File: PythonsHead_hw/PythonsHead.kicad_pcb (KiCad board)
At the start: 2 copper layers, 45 x 79.5 mm, 92 parts, among them Q1 MMBT2222, Q2 MMBT2222, Q3 MMBT2222, Q4 MMBT2222, Q5 MMBT2222, Q6 MMBT2222, Q7 MMBT2222, Q8 MMBT2222

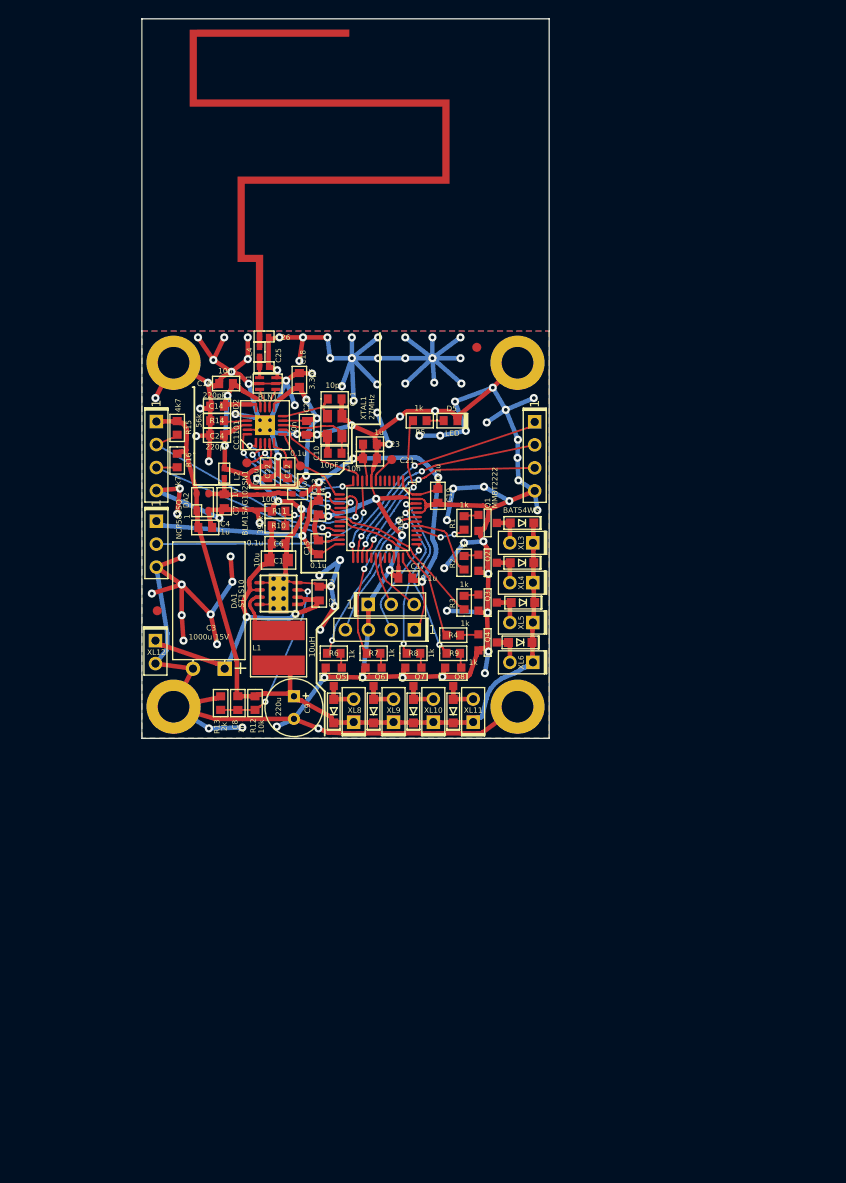
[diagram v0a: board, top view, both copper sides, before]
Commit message: Layout done
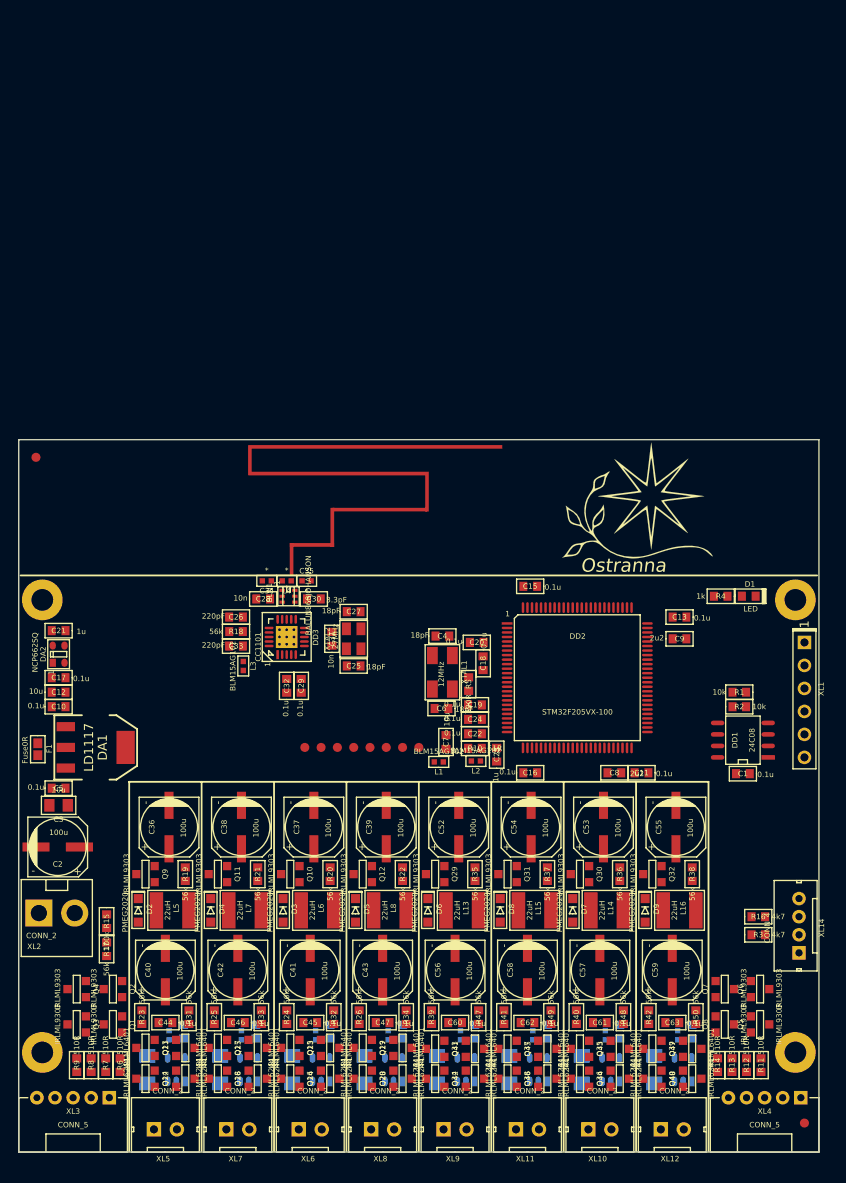
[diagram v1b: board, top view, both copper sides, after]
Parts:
- removed C14: 220pF, Capacitors:CAP_0603
- removed XL13: CONN_3, Connectors:PLS-3
- added C27: 18pF, Capacitors:CAP_0603, F.Cu at (115.4, 85.0)
- added C28: 10n, Capacitors:CAP_0603, F.Cu at (105.4, 83.6)
- added C29: 0.1u, Capacitors:CAP_0603, F.Cu at (109.6, 93.2)
- added C30: 3.3pF, Capacitors:CAP_0603, F.Cu at (111.0, 83.6)
- added C31: 10n, Capacitors:CAP_0603, F.Cu at (113.0, 88.0)
- added C32: 0.1u, Capacitors:CAP_0603, F.Cu at (108.0, 93.2)
- added C33: 220pF, Capacitors:CAP_0603, F.Cu at (102.4, 88.8)
- added C34: *, Capacitors:CAP_0402, F.Cu at (105.8, 81.6)
- added C35: *, Capacitors:CAP_0402, F.Cu at (110.2, 81.6)
- added C36: 100u, Capacitors:SMD_D6d3, F.Cu at (95.0, 108.8)
- added C37: 100u, Capacitors:SMD_D6d3, F.Cu at (111.0, 108.8)
- added C38: 100u, Capacitors:SMD_D6d3, F.Cu at (103.0, 108.8)
- added C39: 100u, Capacitors:SMD_D6d3, F.Cu at (119.0, 108.8)
- added C40: 100u, Capacitors:SMD_D6d3, F.Cu at (94.6, 124.6)
- added C41: 100u, Capacitors:SMD_D6d3, F.Cu at (110.6, 124.6)
- added C42: 100u, Capacitors:SMD_D6d3, F.Cu at (102.6, 124.6)
- added C43: 100u, Capacitors:SMD_D6d3, F.Cu at (118.6, 124.6)
- added C44: 0.1u, Capacitors:CAP_0603, F.Cu at (94.6, 130.4)
- added C45: 0.1u, Capacitors:CAP_0603, F.Cu at (110.6, 130.4)
- added C46: 0.1u, Capacitors:CAP_0603, F.Cu at (102.6, 130.4)
- added C47: 0.1u, Capacitors:CAP_0603, F.Cu at (118.6, 130.4)
- added C48: 0.1u, Capacitors:CAP_0603, B.Cu at (96.6, 131.4)
- added C49: 0.1u, Capacitors:CAP_0603, B.Cu at (112.8, 131.4)
- added C5: 0.1u, Capacitors:CAP_0603, F.Cu at (82.8, 104.5)
- added C50: 0.1u, Capacitors:CAP_0603, B.Cu at (104.6, 131.4)
- added C51: 0.1u, Capacitors:CAP_0603, B.Cu at (120.8, 131.4)
- added C52: 100u, Capacitors:SMD_D6d3, F.Cu at (127.0, 108.8)
- added C53: 100u, Capacitors:SMD_D6d3, F.Cu at (143.0, 108.8)
- added C54: 100u, Capacitors:SMD_D6d3, F.Cu at (135.0, 108.8)
- added C55: 100u, Capacitors:SMD_D6d3, F.Cu at (151.0, 108.8)
- added C56: 100u, Capacitors:SMD_D6d3, F.Cu at (126.6, 124.6)
- added C57: 100u, Capacitors:SMD_D6d3, F.Cu at (142.6, 124.6)
- added C58: 100u, Capacitors:SMD_D6d3, F.Cu at (134.6, 124.6)
- added C59: 100u, Capacitors:SMD_D6d3, F.Cu at (150.6, 124.6)
- added C60: 0.1u, Capacitors:CAP_0603, F.Cu at (126.6, 130.4)
- added C61: 0.1u, Capacitors:CAP_0603, F.Cu at (142.6, 130.4)
- added C62: 0.1u, Capacitors:CAP_0603, F.Cu at (134.6, 130.4)
- added C63: 0.1u, Capacitors:CAP_0603, F.Cu at (150.6, 130.4)
- added C64: 0.1u, Capacitors:CAP_0603, B.Cu at (128.8, 131.4)
- added C65: 0.1u, Capacitors:CAP_0603, B.Cu at (144.8, 131.4)
- added C66: 0.1u, Capacitors:CAP_0603, B.Cu at (136.8, 131.4)
- added C67: 0.1u, Capacitors:CAP_0603, B.Cu at (152.8, 131.4)
- added DA10: AD8211, SOT:SOT23-5, B.Cu at (151.8, 135.6)
- added DA3: AD8211, SOT:SOT23-5, B.Cu at (95.8, 135.6)
- added DA4: AD8211, SOT:SOT23-5, B.Cu at (111.8, 135.6)
- added DA5: AD8211, SOT:SOT23-5, B.Cu at (103.8, 135.6)
- added DA6: AD8211, SOT:SOT23-5, B.Cu at (119.8, 135.6)
- added DA7: AD8211, SOT:SOT23-5, B.Cu at (127.8, 135.6)
- added DA8: AD8211, SOT:SOT23-5, B.Cu at (143.8, 135.6)
- added DA9: AD8211, SOT:SOT23-5, B.Cu at (135.8, 135.6)
- added DD3: CC1101, QFN_DFN:QFN20, F.Cu at (108.0, 87.8)
- added F1: Fuse0R, Resistors:RES_0603_FUSE, F.Cu at (80.5, 100.2)
- added L10: BLM15AG102, Inductors:IND_0402, B.Cu at (111.2, 131.8)
- added L11: BLM15AG102, Inductors:IND_0402, B.Cu at (103.0, 131.8)
- added L12: BLM15AG102, Inductors:IND_0402, B.Cu at (119.2, 131.8)
- added L13: 22uH, Inductors:SRN5040, F.Cu at (127.4, 118.0)
- added L14: 22uH, Inductors:SRN5040, F.Cu at (143.4, 118.0)
- added L15: 22uH, Inductors:SRN5040, F.Cu at (135.4, 118.0)
- added L16: 22uH, Inductors:SRN5040, F.Cu at (151.4, 118.0)
- added L17: BLM15AG102, Inductors:IND_0402, B.Cu at (127.2, 131.8)
- added L18: BLM15AG102, Inductors:IND_0402, B.Cu at (143.2, 131.8)
- added L19: BLM15AG102, Inductors:IND_0402, B.Cu at (135.2, 131.8)
- added L20: BLM15AG102, Inductors:IND_0402, B.Cu at (151.2, 131.8)
- added L5: 22uH, Inductors:SRN5040, F.Cu at (95.4, 118.0)
- added L6: 22uH, Inductors:SRN5040, F.Cu at (111.4, 118.0)
- added L7: 22uH, Inductors:SRN5040, F.Cu at (103.4, 118.0)
- added L8: 22uH, Inductors:SRN5040, F.Cu at (119.4, 118.0)
- added L9: BLM15AG102, Inductors:IND_0402, B.Cu at (95.0, 131.8)
- added Logo1: Logo, Pictures:Ostranna_16d9_13d5, F.Cu at (146.7, 72.7)
- added Q10: IRLML9303, SOT:SOT23-3, F.Cu at (108.4, 114.0)
- added Q11: IRLML9303, SOT:SOT23-3, F.Cu at (100.4, 114.0)
- added Q12: IRLML9303, SOT:SOT23-3, F.Cu at (116.4, 114.0)
- added Q13: IRLML6401, SOT:SOT23-3, F.Cu at (92.4, 133.2)
- added Q14: IRLML6244, SOT:SOT23-3, F.Cu at (92.4, 136.6)
- added Q15: IRLML6401, SOT:SOT23-3, F.Cu at (108.4, 133.2)
- added Q16: IRLML6244, SOT:SOT23-3, F.Cu at (108.4, 136.6)
- added Q17: IRLML6401, SOT:SOT23-3, F.Cu at (100.4, 133.2)
- added Q18: IRLML6244, SOT:SOT23-3, F.Cu at (100.4, 136.6)
- added Q19: IRLML6401, SOT:SOT23-3, F.Cu at (116.4, 133.2)
- added Q20: IRLML6244, SOT:SOT23-3, F.Cu at (116.4, 136.6)
- added Q21: IRLML6401, SOT:SOT23-3, F.Cu at (96.8, 133.2)
- added Q22: IRLML6244, SOT:SOT23-3, F.Cu at (96.8, 136.6)
- added Q23: IRLML6401, SOT:SOT23-3, F.Cu at (112.8, 133.2)
- added Q24: IRLML6244, SOT:SOT23-3, F.Cu at (112.8, 136.6)
- added Q25: IRLML6401, SOT:SOT23-3, F.Cu at (104.8, 133.2)
- added Q26: IRLML6244, SOT:SOT23-3, F.Cu at (104.8, 136.6)
- added Q27: IRLML6401, SOT:SOT23-3, F.Cu at (120.8, 133.2)
- added Q28: IRLML6244, SOT:SOT23-3, F.Cu at (120.8, 136.6)
- added Q29: IRLML9303, SOT:SOT23-3, F.Cu at (124.4, 114.0)
- added Q30: IRLML9303, SOT:SOT23-3, F.Cu at (140.4, 114.0)
- added Q31: IRLML9303, SOT:SOT23-3, F.Cu at (132.4, 114.0)
- added Q32: IRLML9303, SOT:SOT23-3, F.Cu at (148.4, 114.0)
- added Q33: IRLML6401, SOT:SOT23-3, F.Cu at (124.4, 133.3)
- added Q34: IRLML6244, SOT:SOT23-3, F.Cu at (124.4, 136.6)
- added Q35: IRLML6401, SOT:SOT23-3, F.Cu at (140.4, 133.3)
- added Q36: IRLML6244, SOT:SOT23-3, F.Cu at (140.4, 136.6)
- added Q37: IRLML6401, SOT:SOT23-3, F.Cu at (132.4, 133.3)
- added Q38: IRLML6244, SOT:SOT23-3, F.Cu at (132.4, 136.6)
- added Q39: IRLML6401, SOT:SOT23-3, F.Cu at (148.4, 133.3)
- added Q40: IRLML6244, SOT:SOT23-3, F.Cu at (148.4, 136.6)
- added Q41: IRLML6401, SOT:SOT23-3, F.Cu at (128.8, 133.3)
- added Q42: IRLML6244, SOT:SOT23-3, F.Cu at (128.8, 136.6)
- added Q43: IRLML6401, SOT:SOT23-3, F.Cu at (144.8, 133.3)
- added Q44: IRLML6244, SOT:SOT23-3, F.Cu at (144.8, 136.6)
- added Q45: IRLML6401, SOT:SOT23-3, F.Cu at (136.8, 133.3)
- added Q46: IRLML6244, SOT:SOT23-3, F.Cu at (136.8, 136.6)
- added Q47: IRLML6401, SOT:SOT23-3, F.Cu at (152.8, 133.3)
- added Q48: IRLML6244, SOT:SOT23-3, F.Cu at (152.8, 136.6)
- added Q9: IRLML9303, SOT:SOT23-3, F.Cu at (92.4, 114.0)
- added R17: 56k, Resistors:RES_0603, F.Cu at (88.1, 122.3)
- added R18: 56k, Resistors:RES_0603, F.Cu at (102.4, 87.2)
- added R19: 56k, Resistors:RES_0603, F.Cu at (96.8, 114.0)
- added R20: 56k, Resistors:RES_0603, F.Cu at (112.8, 114.0)
- added R21: 56k, Resistors:RES_0603, F.Cu at (104.8, 114.0)
- added R22: 56k, Resistors:RES_0603, F.Cu at (120.8, 114.0)
- added R23: 56k, Resistors:RES_0603, F.Cu at (92.0, 129.8)
- added R24: 56k, Resistors:RES_0603, F.Cu at (108.0, 129.8)
- added R25: 56k, Resistors:RES_0603, F.Cu at (100.0, 129.8)
- added R26: 56k, Resistors:RES_0603, F.Cu at (116.0, 129.8)
- added R27: 0R1, Resistors:RES_1206, B.Cu at (92.6, 135.6)
- added R28: 0R1, Resistors:RES_1206, B.Cu at (108.6, 135.6)
- added R29: 0R1, Resistors:RES_1206, B.Cu at (100.7, 135.6)
- added R30: 0R1, Resistors:RES_1206, B.Cu at (116.6, 135.6)
- added R31: 56k, Resistors:RES_0603, F.Cu at (97.2, 129.8)
- added R32: 56k, Resistors:RES_0603, F.Cu at (113.2, 129.8)
- added R33: 56k, Resistors:RES_0603, F.Cu at (105.2, 129.8)
- added R34: 56k, Resistors:RES_0603, F.Cu at (121.2, 129.8)
- added R35: 56k, Resistors:RES_0603, F.Cu at (128.8, 114.0)
- added R36: 56k, Resistors:RES_0603, F.Cu at (144.8, 114.0)
- added R37: 56k, Resistors:RES_0603, F.Cu at (136.8, 114.0)
- added R38: 56k, Resistors:RES_0603, F.Cu at (152.8, 114.0)
- added R39: 56k, Resistors:RES_0603, F.Cu at (124.0, 129.8)
- added R40: 56k, Resistors:RES_0603, F.Cu at (140.0, 129.8)
- added R41: 56k, Resistors:RES_0603, F.Cu at (132.0, 129.8)
- added R42: 56k, Resistors:RES_0603, F.Cu at (148.0, 129.8)
- added R43: 0R1, Resistors:RES_1206, B.Cu at (124.6, 135.6)
- added R44: 0R1, Resistors:RES_1206, B.Cu at (140.6, 135.6)
- added R45: 0R1, Resistors:RES_1206, B.Cu at (132.6, 135.6)
- added R46: 0R1, Resistors:RES_1206, B.Cu at (148.6, 135.6)
- added R47: 56k, Resistors:RES_0603, F.Cu at (129.2, 129.8)
- added R48: 56k, Resistors:RES_0603, F.Cu at (145.2, 129.8)
- added R49: 56k, Resistors:RES_0603, F.Cu at (137.2, 129.8)
- added R50: 56k, Resistors:RES_0603, F.Cu at (153.2, 129.8)
- added TP4: TESTPOINT, PCB:TESTPOINT_1MM, F.Cu at (115.4, 100.0)
- added TP5: TESTPOINT, PCB:TESTPOINT_1MM, F.Cu at (117.2, 100.0)
- added TP6: TESTPOINT, PCB:TESTPOINT_1MM, F.Cu at (120.8, 100.0)
- added TP7: TESTPOINT, PCB:TESTPOINT_1MM, F.Cu at (119.0, 100.0)
- added TP8: TESTPOINT, PCB:TESTPOINT_1MM, F.Cu at (122.6, 100.0)
- added XTAL2: 27MHz, Quartz:03225C4, F.Cu at (115.4, 88.0)
- ANT1: footprint Radio:ANT_868_MEANDER_4HOR_45mm -> Radio:ANT_868_ARMLETG
- BLN1: value 0896BM15A0001 -> BALUN868JOHANSON
- C1: value 10u -> 0.1u; footprint Capacitors:CAP_0805 -> Capacitors:CAP_0603
- C10, C11: value 10pF -> 0.1u
- C12: value 0.1u -> 10u
- C13: value 4.7u -> 0.1u
- C16, C20: value 10n -> 0.1u
- C18: value 3.3pF -> 0.1u
- C2: value 1u -> 100u; footprint Capacitors:CAP_0603 -> Capacitors:SMD_D6d3
- C21: value 10n -> 1u
- C24: value 220pF -> 0.1u
- C25: value 1.5pF -> 18pF; footprint Capacitors:CAP_0402 -> Capacitors:CAP_0603
- C26: value DoNotMount -> 220pF; footprint Capacitors:CAP_0402 -> Capacitors:CAP_0603
- C3: value 1000u 15V -> 10u; footprint Capacitors:CAP_08xxR_HOR -> Capacitors:CAP_0805
- C4: value 1u -> 18pF
- C6: value 0.1u -> 18pF
- C7: value 1u -> 10u
- C8: value 1n -> 2u2
- C9: value 220u -> 2u2; footprint Capacitors:CAP_06xxR -> Capacitors:CAP_0603
- D1: value BAT54WS -> LED; footprint Diodes:SOD323 -> LEDs:LED_0603
- D2, D3, D4, D6, D7, D8, D9: value BAT54WS -> PMEG2020
- D5: value LED -> PMEG2020; footprint LEDs:LED_0603 -> Diodes:SOD323
- DA1: value ST1S10 -> LD1117; footprint QFN_DFN:DFN8 -> SOT:SOT223
- DA2: value NCP583SQ -> NCP662SQ
- DD1: value STM32L151CxTx -> 24C08; footprint LQFP_TQFP:LQFP48 -> SO_DIL_TSSOP:SO8_150MIL
- DD2: value CC1101 -> STM32F205VX-100; footprint QFN_DFN:QFN20 -> LQFP_TQFP:LQFP100
- HOLE1, HOLE2, HOLE3, HOLE4: footprint PCB:Hole3_5_out6mm -> PCB:Hole2d4_out4d5mm
- L1: value 10uH -> BLM15AG102; footprint Inductors:IND_SDR0604 -> Inductors:IND_0402
- L2, L3: value BLM15AG102SN1 -> BLM15AG102
- L4: value 5.6nH -> *
- Q1, Q2, Q3, Q4, Q5, Q6, Q7, Q8: value MMBT2222 -> IRLML9303
- R1, R2: value 1k -> 10k
- R10: value 390k -> 51R
- R11: value 100k -> 510R
- R12: value 10k -> 510R
- R13: value 2k -> 510R
- R14: value 56k -> 510R
- R15: value 4k7 -> 100k
- R3: value 1k -> 4k7
- R5: value 1k -> 390R
- R6, R7, R8, R9: value 1k -> 510R
- XL1: value CONN_3 -> CONN_6; footprint Connectors:PLS-3 -> Connectors:PLS-6
- XL10, XL11, XL12, XL5, XL6, XL8, XL9: footprint Connectors:PLS-2 -> Connectors:W02_Pitch_2d54
- XL14: footprint Connectors:PLS-4 -> Connectors:WB-04(MW-4M)
- XL2: value ST_SWD -> CONN_2; footprint Connectors:PLS-4 -> Connectors:PWL2-02
- XL3, XL4: value CONN_2 -> CONN_5; footprint Connectors:PLS-2 -> Connectors:WB-05R(MW-5MR)
- XL7: value CONN_4 -> CONN_2; footprint Connectors:PLS-4 -> Connectors:W02_Pitch_2d54
- XTAL1: value 27MHz -> 12MHz; footprint Quartz:03225C4 -> Quartz:0503x4-4
- moved HOLE1 102.6 mm to (164.2, 133.7)
- moved RP1 91.2 mm to (165.2, 141.5)
- moved XL14 90.2 mm to (164.6, 119.7), turned to 90 degrees
- moved R14 90.2 mm to (155.6, 135.1), turned to 90 degrees
- moved XL7 84.8 mm to (102.6, 142.2), turned to 0 degrees
- moved R16 81.6 mm to (160.1, 118.7), turned to 0 degrees
- moved R11 81.2 mm to (160.4, 135.1), turned to 90 degrees
- moved XL3 79.6 mm to (84.4, 138.7)
- moved XL12 78.6 mm to (150.6, 142.2), turned to 0 degrees
- moved R13 69.2 mm to (157.2, 135.1)
- moved XL5 69.2 mm to (94.6, 142.2), turned to 0 degrees
- moved Q1 69.2 mm to (88.8, 130.6), turned to 270 degrees
- moved R12 67.4 mm to (158.8, 135.1), turned to 90 degrees
- moved Q3 65.1 mm to (84.8, 130.6), turned to 270 degrees
- moved HOLE3 64.9 mm to (81.0, 133.7)
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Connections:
- C1 pad 1: +BATT -> GND
- C1 pad 2: GND -> PwrMCU
- C10 pad 1: Net-(C10-Pad1) -> GND
- C10 pad 2: GND -> +5V
- C11 pad 1: Net-(C11-Pad1) -> GND
- C11 pad 2: GND -> PwrMCU
- C12 pad 1: Net-(C12-Pad1) -> GND
- C12 pad 2: GND -> +5V
- C13 pad 1: PwrMCU -> GND
- C13 pad 2: GND -> PwrMCU
- C15 pad 1: PwrMCU -> GND
- C15 pad 2: GND -> PwrMCU
- C16 pad 1: VCC -> GND
- C16 pad 2: GND -> PwrMCU
- C17 pad 1: PwrMCU -> +5V
- C18 pad 1: VCC -> GND
- C18 pad 2: GND -> PwrMCU
- C19 pad 1: PwrMCU -> GND
- C19 pad 2: GND -> PwrMCU
- C2 pad 2: GND -> GNDPWR
- C20 pad 1: VCC -> GND
- C20 pad 2: GND -> PwrMCU
- C21 pad 1: PwrMCU -> +3.3V
- C22 pad 1: VCC -> GND
- C22 pad 2: GND -> /VDDA
- C23 pad 1: PwrMCU -> GND
- C23 pad 2: GND -> /VDDA
- C24 pad 1: VCC -> GND
- C24 pad 2: GND -> /Vref+
- C25 pad 1: /ANT1 -> Net-(C25-Pad1)
- C26 pad 1: /ANT2 -> GND
- C26 pad 2: GND -> VCC
- C3 pad 2: GND -> GNDPWR
- C4 pad 1: +5V -> Net-(C4-Pad1)
- C6 pad 1: GND -> Net-(C6-Pad1)
- C6 pad 2: +BATT -> GND
- C7 pad 1: +3.3V -> GND
- C7 pad 2: GND -> PwrMCU
- C8 pad 1: +5V -> Net-(C8-Pad1)
- C8 pad 2: Net-(C8-Pad2) -> GND
- C9 pad 1: +5V -> Net-(C9-Pad1)
- D1 pad A: /PWM1_OUT -> Net-(D1-PadA)
- D1 pad C: +5V -> GND
- D2 pad A: /PWM2_OUT -> GNDPWR
- D2 pad C: +5V -> Net-(D2-PadC)
- D3 pad A: /PWM3_OUT -> GNDPWR
- D3 pad C: +5V -> Net-(D3-PadC)
- D4 pad A: /PWM4_OUT -> GNDPWR
- D4 pad C: +5V -> Net-(D4-PadC)
- D5 pad A: Net-(D5-PadA) -> GNDPWR
- D5 pad C: GND -> Net-(D5-PadC)
- D6 pad A: /PWM5_OUT -> GNDPWR
- D6 pad C: +5V -> Net-(D6-PadC)
- D7 pad A: /PWM6_OUT -> GNDPWR
- D7 pad C: +5V -> Net-(D7-PadC)
- D8 pad A: /PWM7_OUT -> GNDPWR
- D8 pad C: +5V -> Net-(D8-PadC)
- D9 pad A: /PWM8_OUT -> GNDPWR
- D9 pad C: +5V -> Net-(D9-PadC)
- DA1 pad 1: +BATT -> GND
- DA1 pad 2: +BATT -> +5V
- DA1 pad 3: Net-(C8-Pad2) -> +BATT
- DA1 pad PAD: GND -> +5V
- DA2 pad 1: +5V -> GND
- DA2 pad 2: GND -> +5V
- DD1 pad 1: PwrMCU -> GND
- DD1 pad 2: (no net) -> GND
- DD1 pad 3: (no net) -> GND
- DD1 pad 4: (no net) -> GND
- DD1 pad 5: (no net) -> /SDA_EE
- DD1 pad 6: (no net) -> /SCL_EE
- DD1 pad 7: Net-(DD1-Pad7) -> GND
- DD1 pad 8: GND -> PwrMCU
- DD2 pad 1: /CC_SCK -> (no net)
- DD2 pad 10: Net-(C11-Pad1) -> GND
- DD2 pad 11: VCC -> PwrMCU
- DD2 pad 12: /RF1 -> Net-(C4-Pad1)
- DD2 pad 13: /RF2 -> Net-(DD2-Pad13)
- DD2 pad 14: VCC -> (no net)
- DD2 pad 15: VCC -> /HTRD_CURR
- DD2 pad 16: GND -> /HTRE_CURR
- DD2 pad 17: Net-(DD2-Pad17) -> /HTRF_CURR
- DD2 pad 18: VCC -> /HTRG_CURR
- DD2 pad 19: GND -> PwrMCU
- DD2 pad 2: /CC_MISO -> (no net)
- DD2 pad 20: /CC_MOSI -> GND
- DD2 pad 3: /CC_GDO2 -> (no net)
- DD2 pad 4: VCC -> (no net)
- DD2 pad 5: Net-(C12-Pad1) -> (no net)
- DD2 pad 6: /CC_GDO0 -> PwrMCU
- DD2 pad 7: /CC_CS -> (no net)
- DD2 pad 8: Net-(C10-Pad1) -> (no net)
- DD2 pad 9: VCC -> (no net)
- L1 pad 1: +5V -> PwrMCU
- L1 pad 2: Net-(DA1-Pad7) -> +3.3V
- L2 pad 1: VCC -> /VDDA
- L2 pad 2: +3.3V -> PwrMCU
- L3 pad 1: PwrMCU -> VCC
- Q1 pad 1: Net-(Q1-Pad1) -> /LED1_PWM_CTRL
- Q1 pad 2: GND -> +5V
- Q1 pad 3: /PWM1_OUT -> Net-(Q1-Pad3)
- Q2 pad 1: Net-(Q2-Pad1) -> /LED2_PWM_CTRL
- Q2 pad 2: GND -> +5V
- Q2 pad 3: /PWM2_OUT -> Net-(Q2-Pad3)
- Q3 pad 1: Net-(Q3-Pad1) -> /LED3_PWM_CTRL
- Q3 pad 2: GND -> +5V
- Q3 pad 3: /PWM3_OUT -> Net-(Q3-Pad3)
- Q4 pad 1: Net-(Q4-Pad1) -> /LED4_PWM_CTRL
- Q4 pad 2: GND -> +5V
- Q4 pad 3: /PWM4_OUT -> Net-(Q4-Pad3)
- Q5 pad 1: Net-(Q5-Pad1) -> /LED5_PWM_CTRL
- Q5 pad 2: GND -> +5V
- Q5 pad 3: /PWM5_OUT -> Net-(Q5-Pad3)
- Q6 pad 1: Net-(Q6-Pad1) -> /LED6_PWM_CTRL
- Q6 pad 2: GND -> +5V
- Q6 pad 3: /PWM6_OUT -> Net-(Q6-Pad3)
- Q7 pad 1: Net-(Q7-Pad1) -> /LED7_PWM_CTRL
- Q7 pad 2: GND -> +5V
- Q7 pad 3: /PWM7_OUT -> Net-(Q7-Pad3)
- Q8 pad 1: Net-(Q8-Pad1) -> /LED8_PWM_CTRL
- Q8 pad 2: GND -> +5V
- Q8 pad 3: /PWM8_OUT -> Net-(Q8-Pad3)
- R1 pad 1: /PWM1 -> PwrMCU
- R1 pad 2: Net-(Q1-Pad1) -> /SDA_EE
- R10 pad 1: +BATT -> /Vref+
- R10 pad 2: /BAT_MEAS -> /VDDA
- R11 pad 1: /BAT_MEAS -> Net-(R11-Pad1)
- R11 pad 2: GND -> Net-(Q5-Pad3)
- R12 pad 1: +5V -> Net-(R12-Pad1)
- R12 pad 2: Net-(C8-Pad2) -> Net-(Q6-Pad3)
- R13 pad 1: Net-(C8-Pad2) -> Net-(R13-Pad1)
- R13 pad 2: GND -> Net-(Q7-Pad3)
- R14 pad 1: Net-(DD2-Pad17) -> Net-(R14-Pad1)
- R14 pad 2: GND -> Net-(Q8-Pad3)
- R15 pad 1: +5V -> +BATT
- R15 pad 2: /I2C_SCL -> /BAT_MEAS
- R16 pad 2: /I2C_SDA -> /SDA_SNS
- R2 pad 1: /PWM2 -> /SCL_EE
- R2 pad 2: Net-(Q2-Pad1) -> PwrMCU
- R3 pad 1: /PWM3 -> +5V
- R3 pad 2: Net-(Q3-Pad1) -> /SCL_SNS
- R4 pad 1: /PWM4 -> Net-(D1-PadA)
- R4 pad 2: Net-(Q4-Pad1) -> /LED
- R5 pad 1: Net-(D5-PadA) -> Net-(DD2-Pad13)
- R5 pad 2: Net-(DD1-Pad28) -> Net-(C6-Pad1)
- R6 pad 1: /PWM5 -> Net-(R6-Pad1)
- R6 pad 2: Net-(Q5-Pad1) -> Net-(Q1-Pad3)
- R7 pad 1: /PWM6 -> Net-(R7-Pad1)
- R7 pad 2: Net-(Q6-Pad1) -> Net-(Q2-Pad3)
- R8 pad 1: /PWM7 -> Net-(R8-Pad1)
- R8 pad 2: Net-(Q7-Pad1) -> Net-(Q3-Pad3)
- R9 pad 1: /PWM8 -> Net-(R9-Pad1)
- R9 pad 2: Net-(Q8-Pad1) -> Net-(Q4-Pad3)
- TP1 pad 1: Net-(DD1-Pad7) -> /HTRA_CURR
- TP2 pad 1: /CC_GDO0 -> /HTRC_CURR
- TP3 pad 1: /CC_GDO2 -> /HTRB_CURR
- XL1 pad 1: GND -> PwrMCU
- XL1 pad 2: /UART_TX -> /SWCLK
- XL1 pad 3: /UART_RX -> GND
- XL10 pad 1: +5V -> /HTRG1
- XL10 pad 2: /PWM7_OUT -> /HTRG2
- XL11 pad 1: +5V -> /HTRF1
- XL11 pad 2: /PWM8_OUT -> /HTRF2
- XL12 pad 1: +BATT -> /HTRH1
- XL12 pad 2: GND -> /HTRH2
- XL14 pad 2: /I2C_SCL -> /SCL_SNS
- XL14 pad 3: /I2C_SDA -> /SDA_SNS
- XL2 pad 1: PwrMCU -> GNDPWR
- XL2 pad 2: /SWCLK -> +BATT
- XL3 pad 1: +5V -> GND
- XL3 pad 2: /PWM1_OUT -> Net-(R6-Pad1)
- XL4 pad 1: +5V -> GND
- XL4 pad 2: /PWM2_OUT -> Net-(R11-Pad1)
- XL5 pad 1: +5V -> /HTRA1
- XL5 pad 2: /PWM3_OUT -> /HTRA2
- XL6 pad 1: +5V -> /HTRC1
- XL6 pad 2: /PWM4_OUT -> /HTRC2
- XL7 pad 1: Net-(DD1-Pad25) -> /HTRB1
- XL7 pad 2: Net-(DD1-Pad26) -> /HTRB2
- XL8 pad 1: +5V -> /HTRD1
- XL8 pad 2: /PWM5_OUT -> /HTRD2
- XL9 pad 1: +5V -> /HTRE1
- XL9 pad 2: /PWM6_OUT -> /HTRE2
- XTAL1 pad 1: Net-(C10-Pad1) -> Net-(C4-Pad1)
- XTAL1 pad 2: Net-(C11-Pad1) -> Net-(C6-Pad1)
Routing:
- net GND: track 536.4 -> 0.00 mm, vias 103 -> 0
- net +5V: track 92.4 -> 0.00 mm
- net PwrMCU: track 78.7 -> 0.00 mm, vias 5 -> 0
- net VCC: track 59.8 -> 0.00 mm, vias 5 -> 0
- net +BATT: track 41.6 -> 0.00 mm, vias 2 -> 0
- net Net-(DD1-Pad10): track 27.8 -> 0.00 mm, vias 1 -> 0
- net Net-(DD1-Pad25): track 27.0 -> 0.00 mm, vias 2 -> 0
- net Net-(DD1-Pad26): track 25.3 -> 0.00 mm, vias 2 -> 0
- net /I2C_SCL: track 25.2 -> 0.00 mm, vias 1 -> 0
- net Net-(DD1-Pad27): track 24.2 -> 0.00 mm, vias 2 -> 0
- net /I2C_SDA: track 24.0 -> 0.00 mm, vias 1 -> 0
- net /PWM8: track 19.7 -> 0.00 mm, vias 2 -> 0
- net Net-(C8-Pad2): track 19.5 -> 0.00 mm, vias 2 -> 0
- net /PWM4: track 18.8 -> 0.00 mm
- net /PWM5: track 18.4 -> 0.00 mm, vias 2 -> 0
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- removed copper zone on B.Cu, net GND
- removed copper zone on F.Cu, net GND
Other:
- board size 45 x 79.5 mm -> 88.4 x 78.7 mm
- board text added: "Ostranna"
